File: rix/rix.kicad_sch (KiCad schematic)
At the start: 20 parts, among them J1 9V BAT - +, J2 Detection coil, J3 External antenna, SW1 On/Off SW, U1 74LS04, U2 L78L05_SOT89, Y1 8.0 Mhz Crystal, Y2 8.0 Mhz Crystal

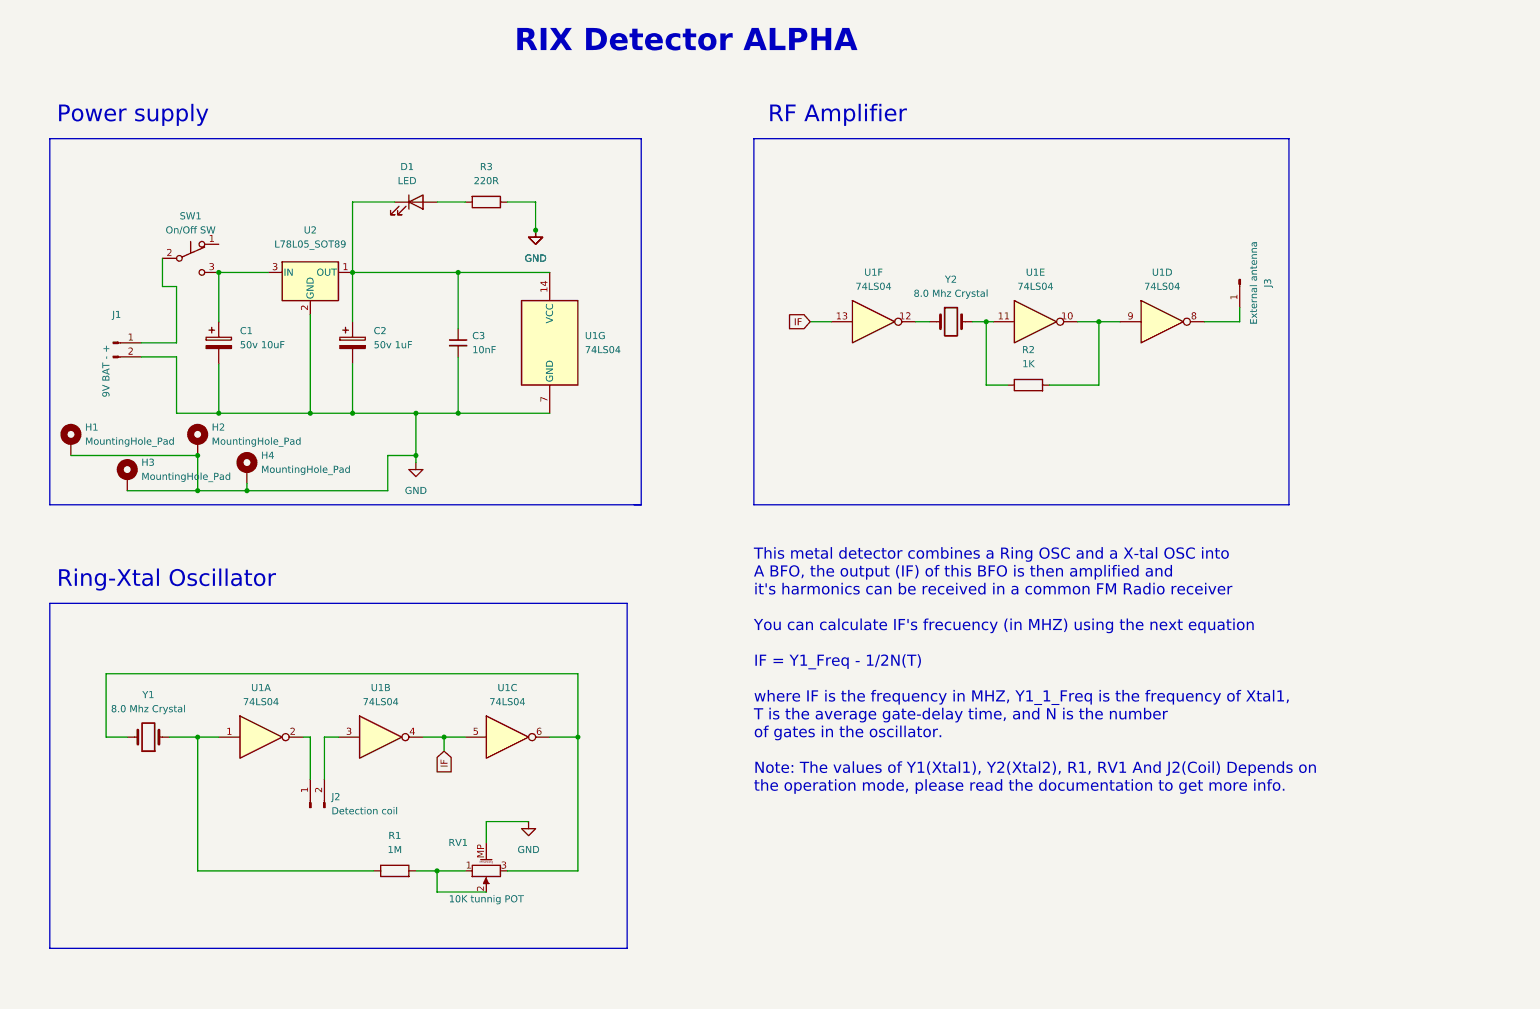
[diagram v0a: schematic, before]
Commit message: Updating gerber files
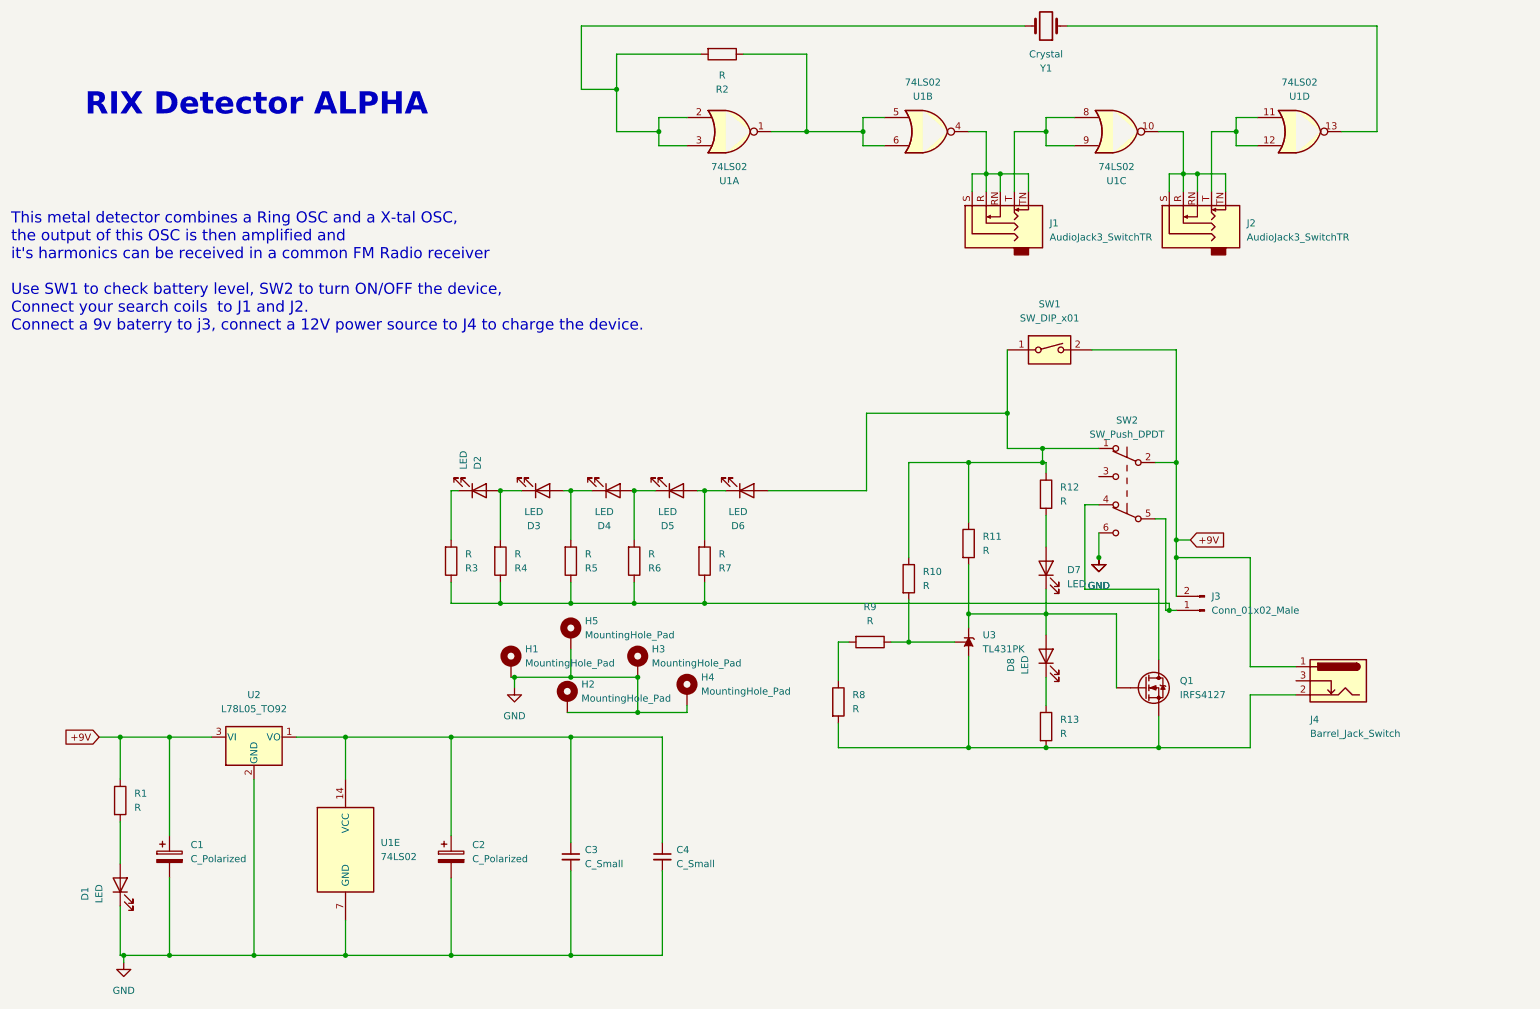
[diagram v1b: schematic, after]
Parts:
- removed J1: 9V BAT - +, Connector_JST:JST_PH_B2B-PH-K_1x02_P2.00mm_Vertical, symbol Connector:Conn_01x02_Male
- removed J2: Detection coil, Connector_PinHeader_2.54mm:PinHeader_1x02_P2.54mm_Vertical, symbol Connector:Conn_01x02_Male
- removed J3: External antenna, Connector_PinHeader_2.54mm:PinHeader_1x01_P2.54mm_Vertical, symbol Connector:Conn_01x01_Male
- removed RV1: 10K tunnig POT, Potentiometer_THT:Potentiometer_Alps_RK09K_Single_Vertical, symbol Device:R_Potentiometer_MountingPin
- removed SW1: On/Off SW, Button_Switch_THT:SW_Push_1P2T_Vertical_E-Switch_800UDP8P1A1M6, symbol Switch:SW_Push_SPDT
- removed U1: 74LS04, Package_SO:SOIC-14_3.9x8.7mm_P1.27mm, symbol 74xx:74LS04
- removed U2: L78L05_SOT89, Package_TO_SOT_SMD:SOT-89-3, symbol Regulator_Linear:L78L05_SOT89
- removed Y2: 8.0 Mhz Crystal, Crystal:Crystal_HC49-4H_Vertical, symbol Device:Crystal
- added C4: C_Small, Capacitor_THT:C_Disc_D3.8mm_W2.6mm_P2.50mm, symbol Device:C_Small
- added D2, D3, D4, D5, D6, D7, D8: LED, LED_THT:LED_D3.0mm, symbol Device:LED
- added H5: MountingHole_Pad, MountingHole:MountingHole_2.2mm_M2_DIN965_Pad_TopBottom, symbol Mechanical:MountingHole_Pad
- added J1, J2: AudioJack3_SwitchTR, Connector_Audio:Jack_3.5mm_Ledino_KB3SPRS_Horizontal, symbol Connector:AudioJack3_SwitchTR
- added J3: Conn_01x02_Male, Connector_JST:JST_XH_B2B-XH-A_1x02_P2.50mm_Vertical, symbol Connector:Conn_01x02_Male
- added J4: Barrel_Jack_Switch, Connector_BarrelJack:BarrelJack_Horizontal, symbol Connector:Barrel_Jack_Switch
- added Q1: IRFS4127, Package_TO_SOT_THT:TO-92_Wide, symbol Transistor_FET:IRFS4127
- added R10, R11, R12, R13, R4, R5, R6, R7, R8, R9: R, Resistor_THT:R_Axial_DIN0204_L3.6mm_D1.6mm_P5.08mm_Horizontal, symbol Device:R
- added SW1: SW_DIP_x01, Button_Switch_THT:SW_PUSH_6mm_H5mm, symbol Switch:SW_DIP_x01
- added SW2: SW_Push_DPDT, Button_Switch_THT:SW_Push_2P2T_Toggle_CK_PVA2OAH5xxxxxxV2, symbol Switch:SW_Push_DPDT
- added U1: 74LS02, Package_DIP:DIP-14_W7.62mm, symbol 74xx:74LS02
- added U2: L78L05_TO92, Package_TO_SOT_THT:TO-92_Wide, symbol Regulator_Linear:L78L05_TO92
- added U3: TL431PK, Package_TO_SOT_THT:TO-92_Wide, symbol Reference_Voltage:TL431PK
- C1: value 50v 10uF -> C_Polarized; footprint Capacitor_THT:CP_Radial_D5.0mm_P2.00mm -> Capacitor_THT:CP_Radial_D6.3mm_P2.50mm
- C2: value 50v 1uF -> C_Polarized; footprint Capacitor_THT:CP_Radial_D5.0mm_P2.00mm -> Capacitor_THT:CP_Radial_D6.3mm_P2.50mm
- C3: value 10nF -> C_Small; footprint Capacitor_SMD:C_0805_2012Metric_Pad1.18x1.45mm_HandSolder -> Capacitor_THT:C_Disc_D3.8mm_W2.6mm_P2.50mm
- D1: footprint Diode_SMD:D_1206_3216Metric_Pad1.42x1.75mm_HandSolder -> LED_THT:LED_D3.0mm
- R1: value 1M -> R; footprint Resistor_SMD:R_0805_2012Metric_Pad1.20x1.40mm_HandSolder -> Resistor_THT:R_Axial_DIN0204_L3.6mm_D1.6mm_P5.08mm_Horizontal
- R2: value 1K -> R; footprint Resistor_SMD:R_0805_2012Metric_Pad1.20x1.40mm_HandSolder -> Resistor_THT:R_Axial_DIN0204_L3.6mm_D1.6mm_P5.08mm_Horizontal
- R3: value 220R -> R; footprint Resistor_SMD:R_0805_2012Metric_Pad1.20x1.40mm_HandSolder -> Resistor_THT:R_Axial_DIN0204_L3.6mm_D1.6mm_P5.08mm_Horizontal
- Y1: value 8.0 Mhz Crystal -> Crystal
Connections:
- net GND: now also D1.1 (K), C4.2, H5.1, SW2.6 (C), U1.7 (GND), U2.2 (GND); no longer R3.1
- net +9V: now reaches C1.1
- net +9V: now also R1.1, J3.2 (Pin_2), J4.1, SW1.2, SW2.2 (B), U2.3 (VI)
- net at R3.2: now also D2.1 (K); no longer D1.2 (A)
- net at C2.1, C3.1: now also C4.1, U1.14 (VCC), U2.1 (VO); no longer D1.1 (K)
- net at Y1.1: now also U1.13; no longer R1.1
- net at R1.2: now also D1.2 (A)
- net at R2.1: now also U1.1, U1.5, U1.6
- net at R2.2: now also Y1.2, U1.2, U1.3
- new net: J3.1 (Pin_1), R3.1, R4.1, R5.1, R6.1, R7.1, SW2.5 (B)
- new net: D2.2 (A), D3.1 (K), R4.2
- new net: J1.R, J1.RN, J1.S, J1.TN, U1.4
- new net: J1.T, U1.8, U1.9
- new net: J4.2, Q1.3 (S), R13.2, R8.2, U3.2 (A)
- new net: D7.1 (K), D8.2 (A), Q1.1 (G), R11.2, U3.3 (K)
- new net: Q1.2 (D), SW2.4 (A)
- new net: D4.2 (A), D5.1 (K), R6.2
- new net: D8.1 (K), R13.1
- new net: D6.2 (A), R10.1, R11.1, R12.1, SW1.1, SW2.1 (A)
- new net: D7.2 (A), R12.2
- new net: R8.1, R9.2
- new net: R10.2, R9.1, U3.1 (REF)
- new net: D5.2 (A), D6.1 (K), R7.2
- new net: J2.T, U1.11, U1.12
- new net: J2.R, J2.RN, J2.S, J2.TN, U1.10
- new net: D3.2 (A), D4.1 (K), R5.2
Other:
- note added: "This metal detector combines a Ring OSC and a X-tal OSC, the output of this OSC is then amplified and it's harmonics can be received in a common FM Radio receiver Use SW1 to check battery level, SW2 to turn ON/OFF the device, Connect your search coils to J1 and J2. Connect a 9v baterry to j3, connect a 12V power source to J4 to charge the device."
- note removed: "Power supply"
- note removed: "RF Amplifier"
- note removed: "Ring-Xtal Oscillator"
- note removed: "This metal detector combines a Ring OSC and a X-tal OSC into A BFO, the output (IF) of this BFO is then amplified and it's harmonics can be received in a common FM Radio receiver You can calculate IF's frecuency (in MHZ) using the next equation IF = Y1_Freq - 1/2N(T) where IF is the frequency in MHZ, Y1_1_Freq is the frequency of Xtal1, T is the average gate-delay time, and N is the number of gat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"
